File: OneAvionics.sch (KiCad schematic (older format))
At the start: 40 parts, among them J1 Conn_01x02, J2 USB_B_Micro, J3 SWD, SW1 SW_SPDT, SW2 SW_SPDT, SW3 SW_Push, U1 STM32F103C8Tx, U3 LM1117-3.3, Y1 16MHz

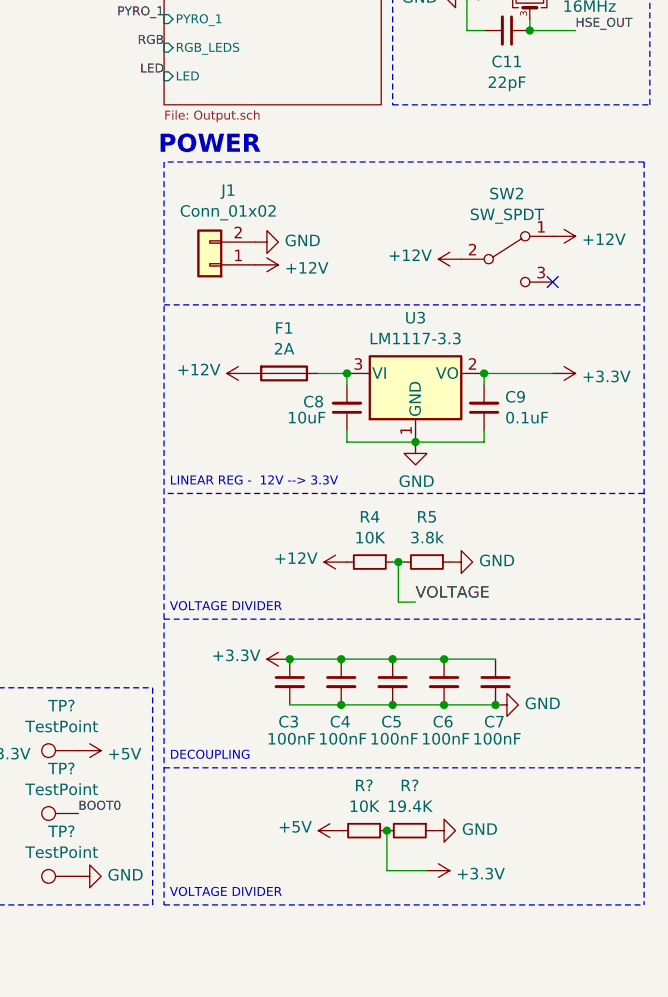
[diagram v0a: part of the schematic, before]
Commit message: rc and cont on pyro, linear reg, flash
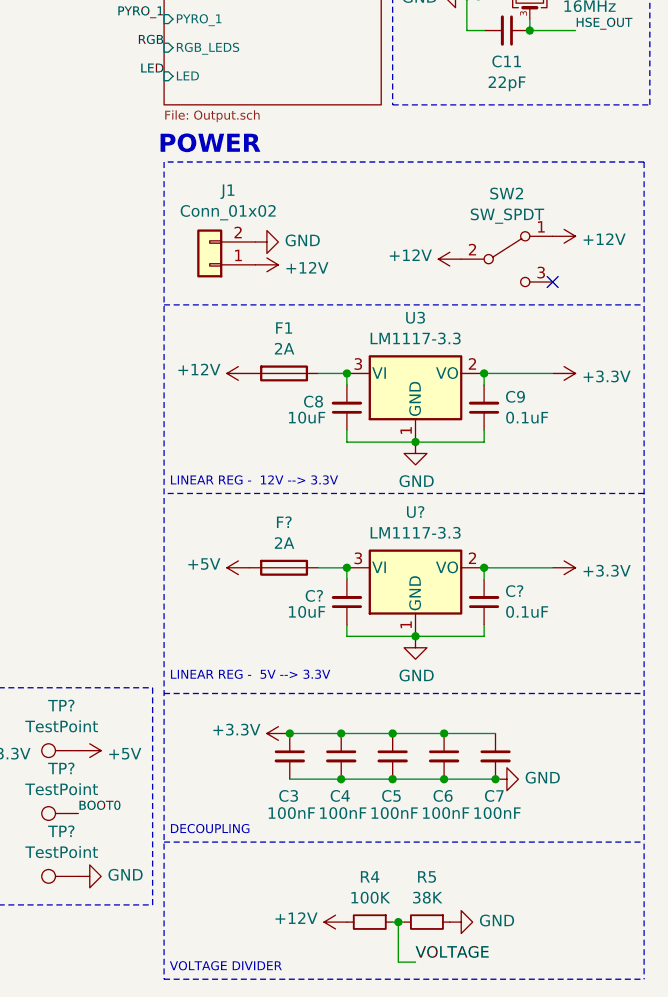
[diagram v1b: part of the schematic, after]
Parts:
- removed R?: 10K, symbol Device:R_Small
- removed R?: 19.4K, symbol Device:R_Small
- added C?: 10uF, Capacitor_SMD:C_0603_1608Metric, symbol Device:C_Small
- added C?: 0.1uF, Capacitor_SMD:C_0603_1608Metric, symbol Device:C_Small
- added F?: 2A, Fuse:Fuse_1206_3216Metric_Castellated, symbol Device:Fuse
- added U?: LM1117-3.3, Package_TO_SOT_SMD:SOT-223, symbol Regulator_Linear:LM1117-3.3
- R4: value 10K -> 100K
- R5: value 3.8k -> 38K
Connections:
- net +3V3: now also C?.2, U?.2 (VO)
- net +5V: now also F?.2
- net GND: now also C?.1, C?.1, U?.1 (GND)
- new net: C?.2, F?.1, U?.3 (VI)
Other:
- note added: "LINEAR REG - 5V --> 3.3V"
- moved on the sheet: C3, C4, C5, C6, C7, R4, R5
